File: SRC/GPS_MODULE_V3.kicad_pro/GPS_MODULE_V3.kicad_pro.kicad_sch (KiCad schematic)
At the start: 11 parts, among them J1 Input, J2 Conn_02x02_Odd_Even, Q1 SSM3J328R-HXY

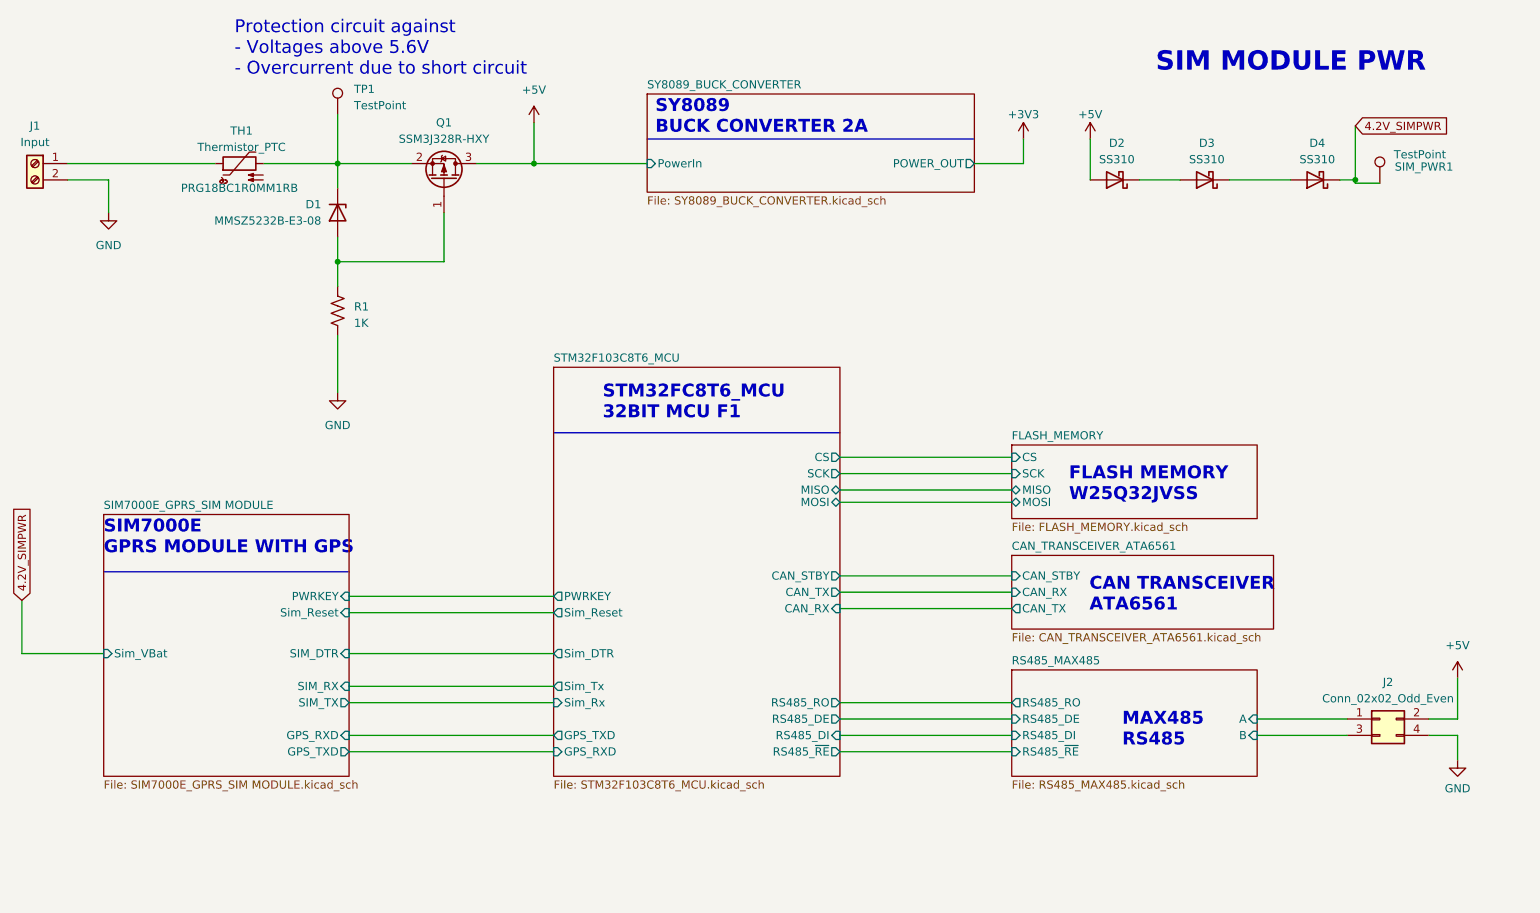
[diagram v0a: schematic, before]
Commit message: updates on BOM, CPL and gerbers
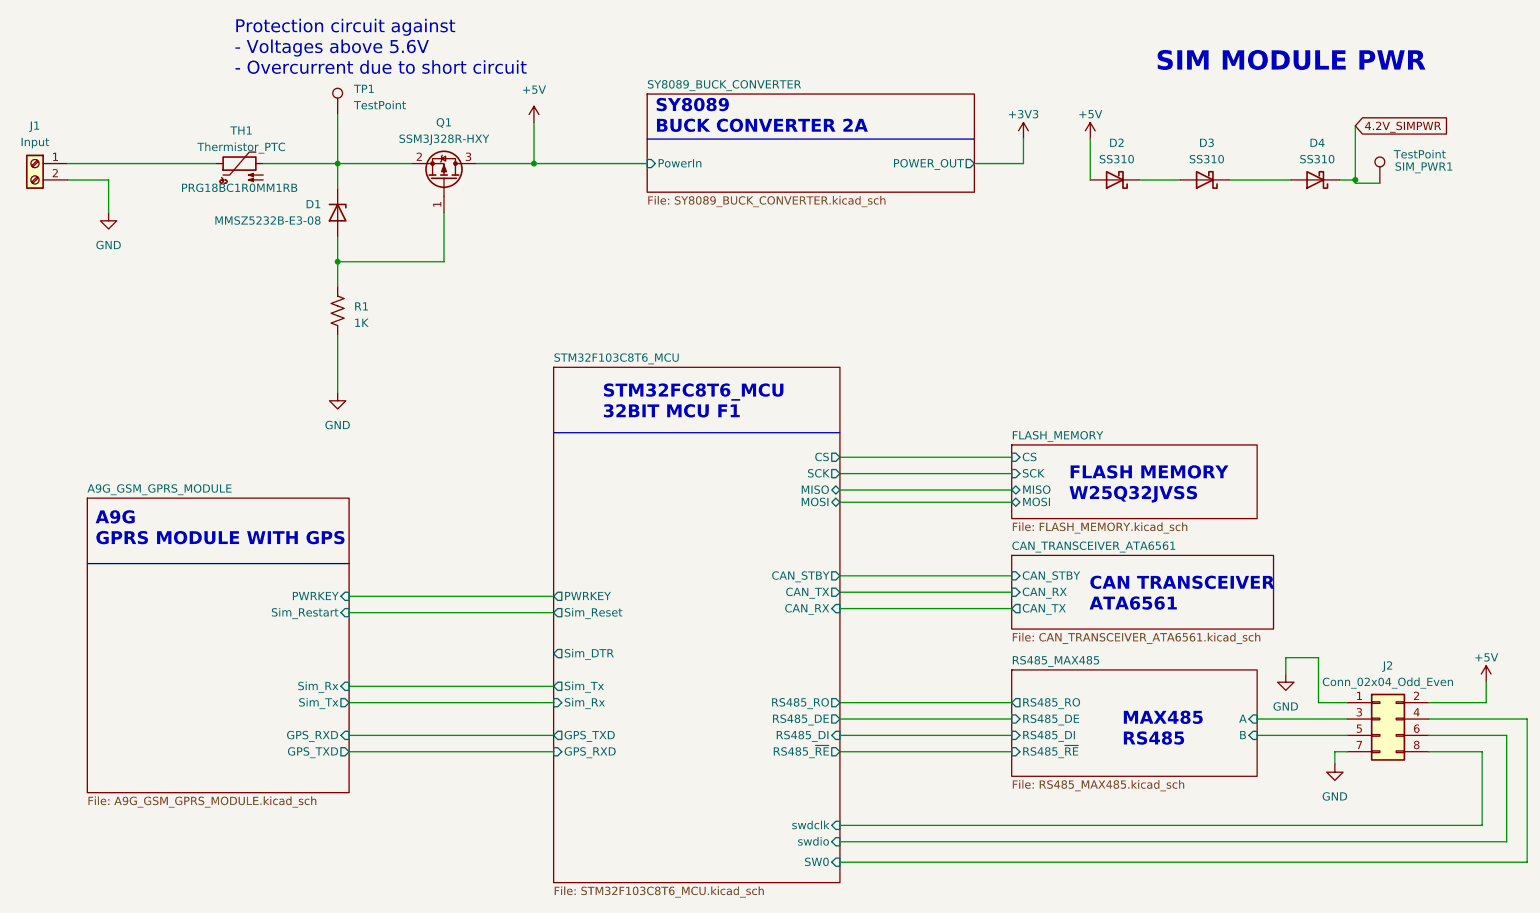
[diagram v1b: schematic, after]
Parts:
- removed J2: Conn_02x02_Odd_Even, Connector_Molex:Molex_Nano-Fit_105314-xx04_2x02_P2.50mm_Horizontal, symbol Connector_Generic:Conn_02x02_Odd_Even
- added J2: Conn_02x04_Odd_Even, Connector_Molex:Molex_Mini-Fit_Jr_5569-08A2_2x04_P4.20mm_Horizontal, symbol Connector_Generic:Conn_02x04_Odd_Even
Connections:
- net +5V: now also J2.2 (Pin_2)
- net GND: now also J2.1 (Pin_1), J2.7 (Pin_7)
- net RS485_MAX485/A: now also J2.3 (Pin_3)
- net RS485_MAX485/B: now also J2.5 (Pin_5)
- new net STM32F103C8T6_MCU/SW0: J2.4 (Pin_4)
- new net STM32F103C8T6_MCU/swdclk: J2.8 (Pin_8)
- new net STM32F103C8T6_MCU/swdio: J2.6 (Pin_6)
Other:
- removed sheet SIM7000E_GPRS_SIM MODULE
- added sheet A9G_GSM_GPRS_MODULE (A9G_GSM_GPRS_MODULE.kicad_sch)
- sheet STM32F103C8T6_MCU ports: added SW0, swdclk, swdio; removed none
- note added: "A9G GPRS MODULE WITH GPS"
- note removed: "SIM7000E GPRS MODULE WITH GPS"
